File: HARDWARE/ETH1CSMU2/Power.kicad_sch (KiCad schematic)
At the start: 40 parts, among them Q1 IRFR5410, U31 MAX5902, U32 TMR 4-2411WI, U33 TEL 12-2423, U34 NCV1117DT33T5G

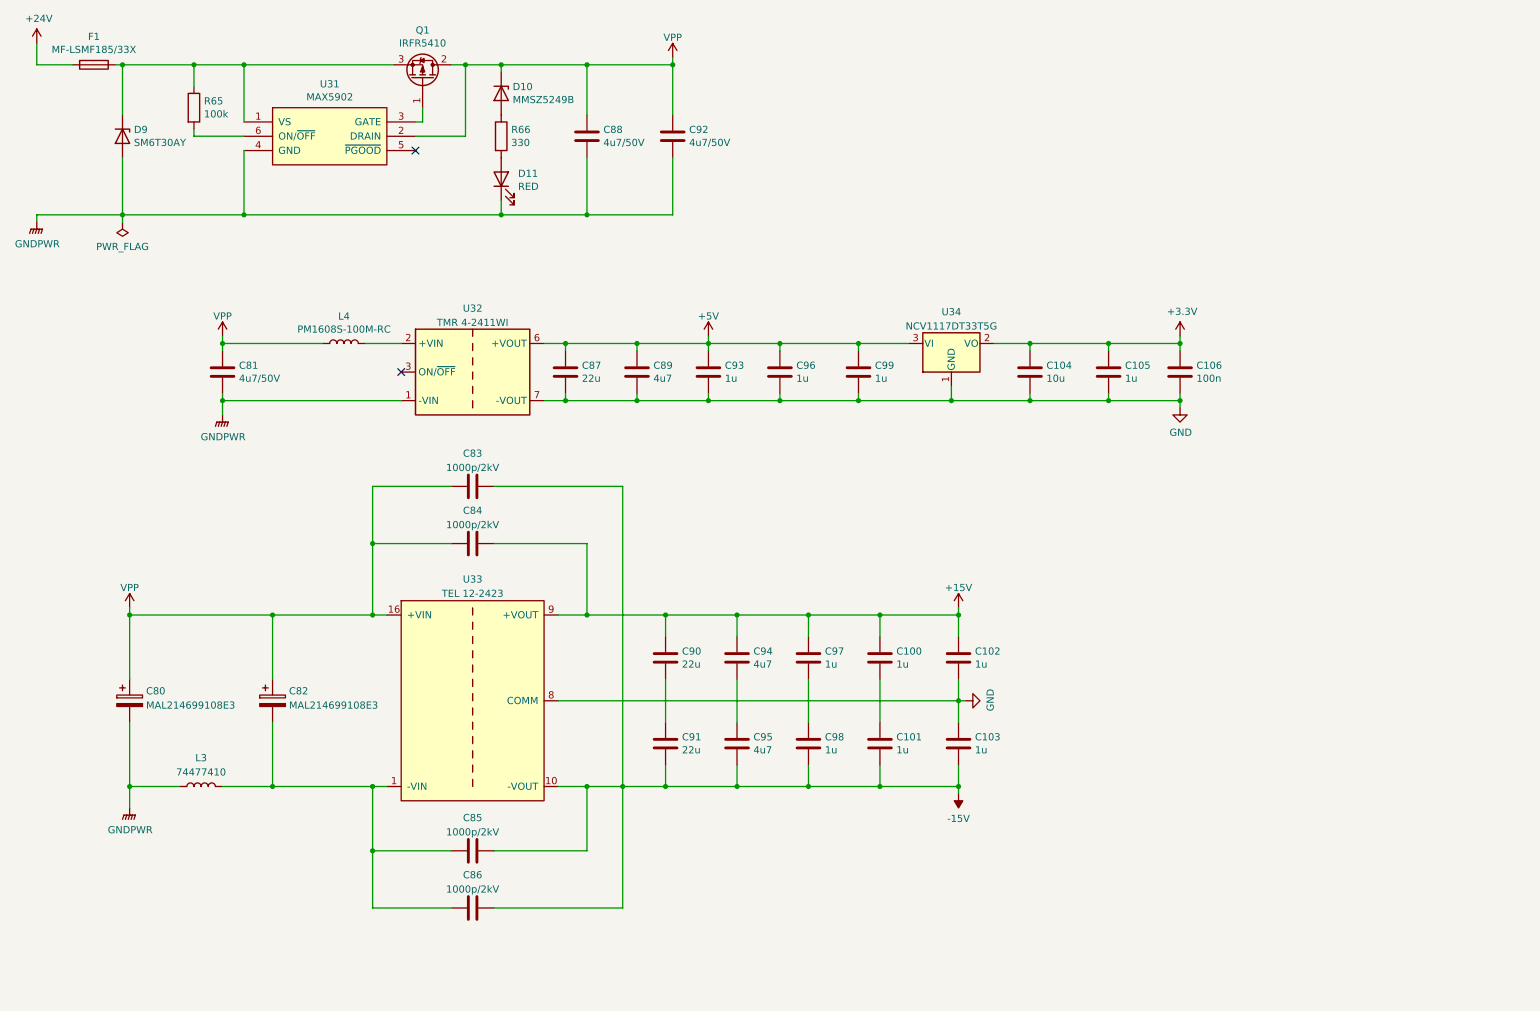
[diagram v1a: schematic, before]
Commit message: Hardware design
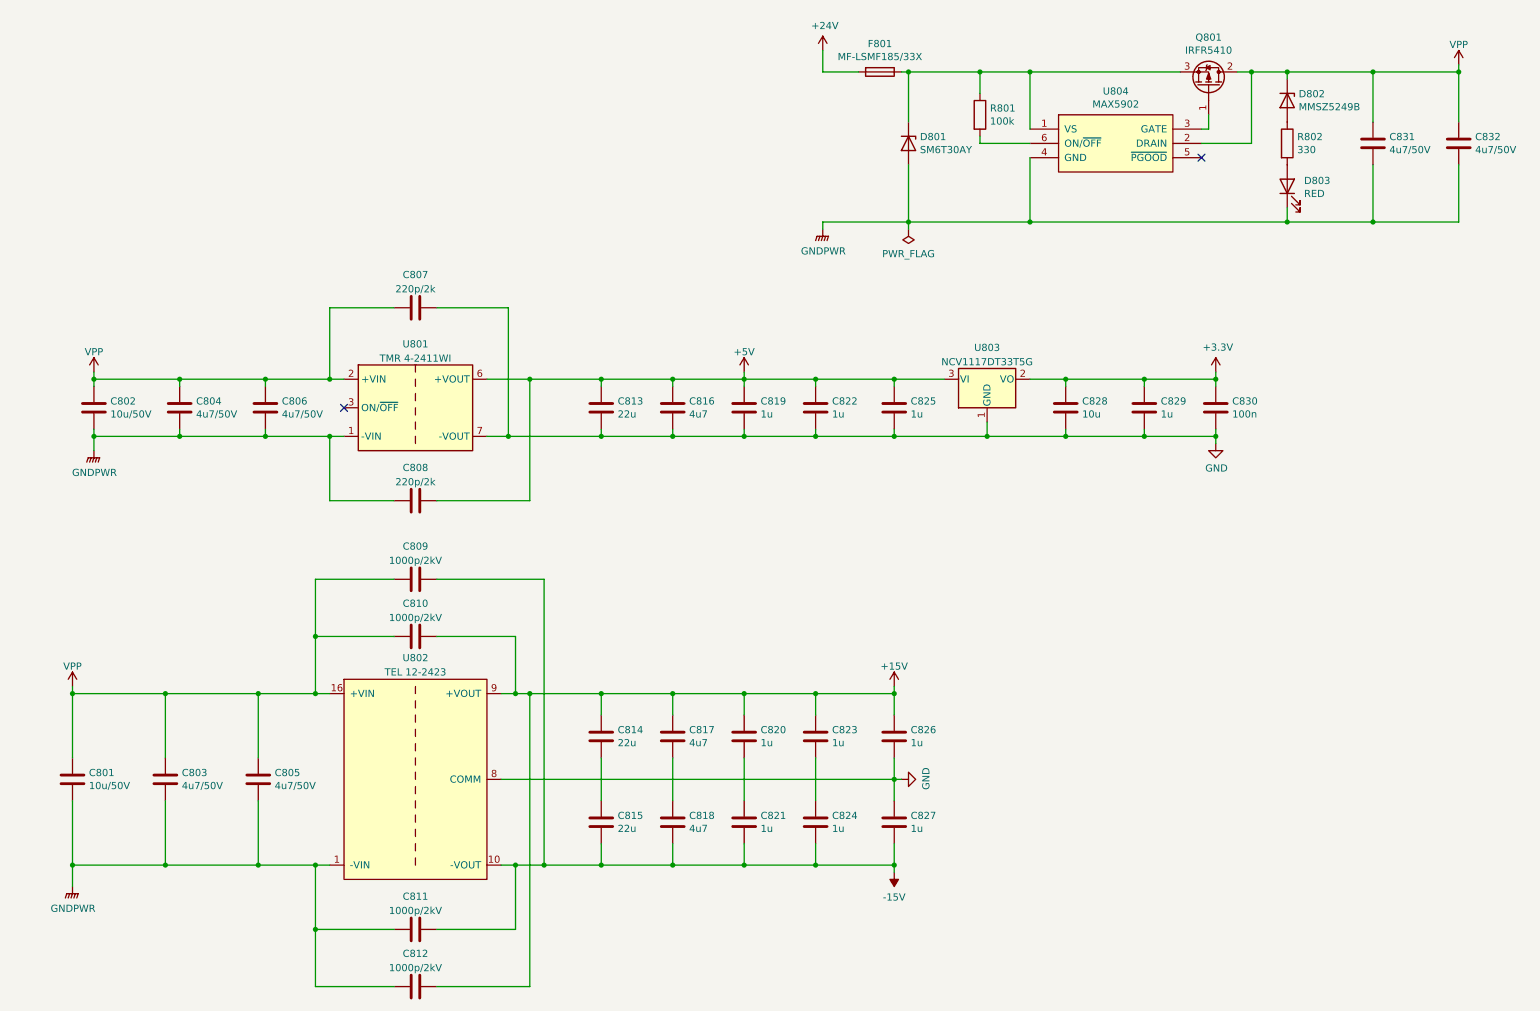
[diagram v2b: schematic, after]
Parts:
- removed C80, C82: MAL214699108E3, Capacitor_SMD:CP_Elec_18x17.5, symbol Device:C_Polarized
- removed L3: 74477410, ETH1CSMU2:74477410, symbol Device:L
- removed L4: PM1608S-100M-RC, ETH1CLCR2:PM1608S, symbol Device:L
- added C801, C802: 10u/50V, Capacitor_SMD:C_1206_3216Metric_Pad1.33x1.80mm_HandSolder, symbol Device:C
- added C803, C804, C805: 4u7/50V, Capacitor_SMD:C_1206_3216Metric_Pad1.33x1.80mm_HandSolder, symbol Device:C
- added C807, C808: 220p/2k, Capacitor_SMD:C_1812_4532Metric_Pad1.57x3.40mm_HandSolder, symbol Device:C
- D801: renamed from D9; footprint ETH1CLCR2:DO_214AA_REV -> ETH1CSMU2:DO_214AA_REV
- F801: renamed from F1; footprint ETH1CLCR2:Fuse_SMD2920 -> ETH1CSMU2:Fuse_SMD2920
- Q801: renamed from Q1; footprint ETH1CLCR2:TO-252-2_Rectifier -> ETH1CSMU2:TO-252-2_Rectifier
- U804: renamed from U31; symbol ETH1CLCR2:MAX5902 -> ETH1CSMU2:MAX5902
- renumbered C81 to C806, C83 to C809, C84 to C810, C85 to C811, C86 to C812, C87 to C813, C90 to C814, C91 to C815, C89 to C816, C94 to C817, C95 to C818, C93 to C819, C97 to C820, C98 to C821, C96 to C822, C100 to C823, C101 to C824, C99 to C825, C102 to C826, C103 to C827, C104 to C828, C105 to C829, C106 to C830, C88 to C831, C92 to C832, D10 to D802, D11 to D803, R65 to R801, R66 to R802, U32 to U801, U33 to U802, U34 to U803
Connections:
- net +15V: now also C812.2
- net +5V: now also C808.2
- net -15V: no longer C812.2
- net GND: now also C807.2
- net GNDPWR: now also C811.1, C812.1, U802.1 (-VIN), C801.2, C802.2, C803.2, C804.2, C805.2, C808.1
- net VPP: now also U801.2 (+VIN), C801.1, C802.1, C803.1, C804.1, C805.1, C807.1
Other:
- moved on the sheet: C806, C809, C810, C811, C812, C813, C814, C815, C816, C817, C818, C819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
